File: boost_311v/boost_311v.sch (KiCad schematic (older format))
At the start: 62 parts, among them J1 Vin_Cnt, J2 VO, J3 Vin_boost, Q1 BC556, Q2 PN2222A, Q5 IRFP260, U1 LM358, U2 L7812, U3 TC4420CPA, U4 LF357, U5 NE555

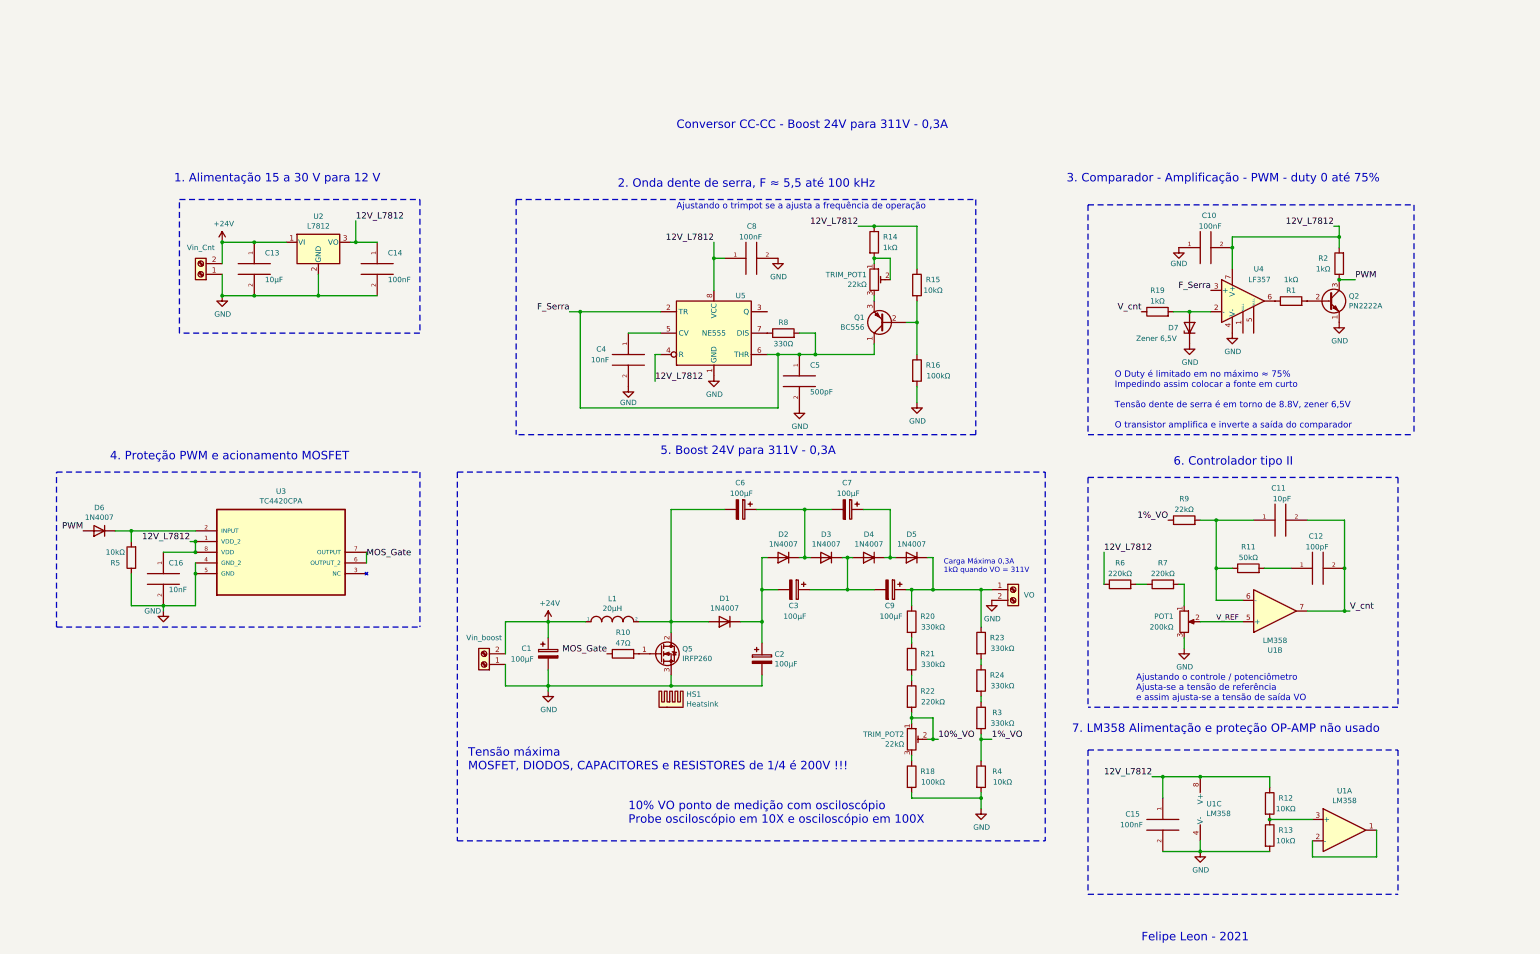
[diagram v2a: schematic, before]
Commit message: UP ocbs
Signed-off-by: fgl27 <fglfgl27@gmail.com>
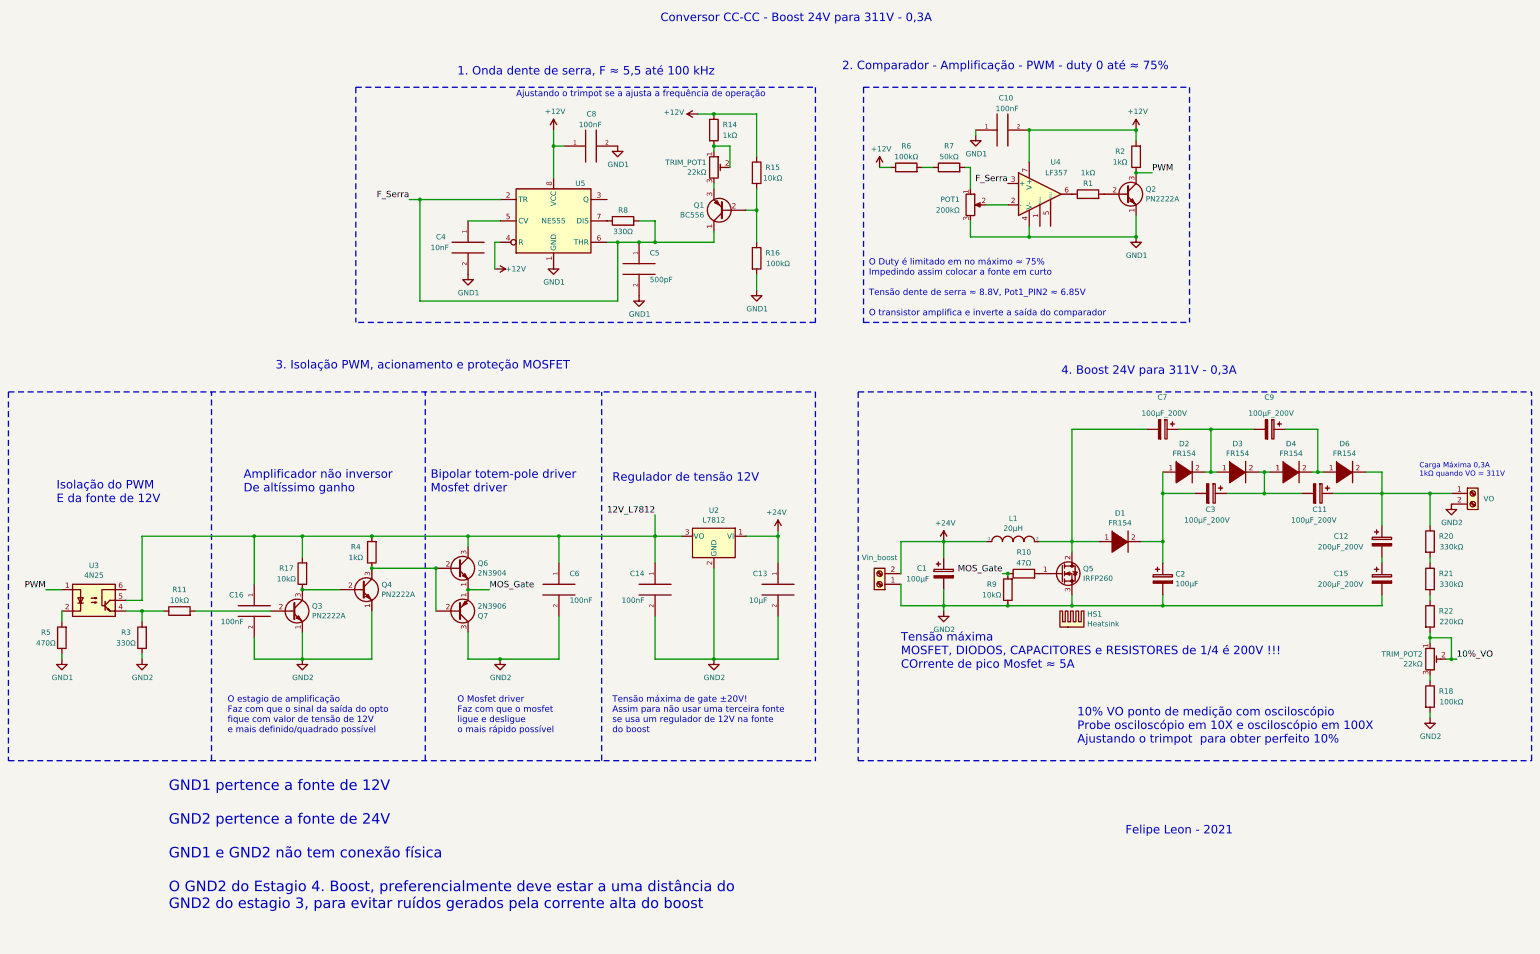
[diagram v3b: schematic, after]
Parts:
- removed C11: 10pF, Capacitor_THT:C_Disc_D7.5mm_W5.0mm_P5.00mm, symbol pspice:CAP
- removed C12: 100pF, Capacitor_THT:C_Disc_D7.5mm_W5.0mm_P5.00mm, symbol pspice:CAP
- removed C15: 100nF, Capacitor_THT:C_Disc_D7.5mm_W5.0mm_P5.00mm, symbol pspice:CAP
- removed C6: 100µF, Capacitor_THT:CP_Radial_D18.0mm_P7.50mm, symbol Device:CP
- removed D1, D2, D3, D4, D5, D6: 1N4007, Diode_THT:D_DO-41_SOD81_P10.16mm_Horizontal, symbol Diode:1N4007
- removed D7: Zener 6,5V, symbol Device:D_Zener
- removed J1: Vin_Cnt, symbol Connector:Screw_Terminal_01x02
- removed R12: 10KΩ, Resistor_THT:R_Axial_DIN0207_L6.3mm_D2.5mm_P10.16mm_Horizontal, symbol Device:R
- removed R13: 10kΩ, Resistor_THT:R_Axial_DIN0207_L6.3mm_D2.5mm_P10.16mm_Horizontal, symbol Device:R
- removed R19: 1kΩ, Resistor_THT:R_Axial_DIN0207_L6.3mm_D2.5mm_P10.16mm_Horizontal, symbol Device:R
- removed R23, R24: 330kΩ, Resistor_THT:R_Axial_DIN0207_L6.3mm_D2.5mm_P10.16mm_Horizontal, symbol Device:R
- removed U1: LM358, symbol Amplifier_Operational:LM358
- removed U3: TC4420CPA, DIP254P762X533-8, symbol 4420:TC4420CPA
- added C11: 100µF_200V, Capacitor_THT:CP_Radial_D18.0mm_P7.50mm, symbol Device:CP
- added C12, C15: 200µF_200V, Capacitor_THT:CP_Radial_D18.0mm_P7.50mm, symbol Device:CP
- added C6: 100nF, Capacitor_THT:C_Disc_D7.5mm_W5.0mm_P5.00mm, symbol pspice:CAP
- added D1, D2, D3, D4, D6: FR154, Diode_THT:D_DO-41_SOD81_P10.16mm_Horizontal, symbol pspice:DIODE
- added Q3, Q4: PN2222A, Package_TO_SOT_THT:TO-92_Inline, symbol Transistor_BJT:PN2222A
- added Q6: 2N3904, Package_TO_SOT_THT:TO-92_Inline, symbol Transistor_BJT:2N3904
- added Q7: 2N3906, Package_TO_SOT_THT:TO-92_Inline, symbol Transistor_BJT:2N3906
- added R17: 10kΩ, Resistor_THT:R_Axial_DIN0207_L6.3mm_D2.5mm_P10.16mm_Horizontal, symbol Device:R
- added U3: 4N25, Package_DIP:DIP-6_W7.62mm, symbol Isolator:4N25
- C16: value 10nF -> 100nF
- C3, C7, C9: value 100µF -> 100µF_200V
- R11: value 50kΩ -> 10kΩ
- R3: value 330kΩ -> 330Ω
- R4: value 10kΩ -> 1kΩ
- R5: value 10kΩ -> 470Ω
- R6: value 220kΩ -> 100kΩ
- R7: value 220kΩ -> 50kΩ
- R9: value 22kΩ -> 10kΩ
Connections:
- net V_REF is gone; now on an unnamed net: POT1.2
- net 12V_L7812: now also R4.2, C6.1, Q6.3 (C), R17.2, U3.5; no longer C10.2, C8.1, R14.1, R15.1, R2.2, R6.1, U4.7 (V+), U5.4 (R), U5.8 (VCC)
- net MOS_Gate: now also R9.2, Q6.1 (E), Q7.1 (E)
- net PWM: now also U3.1
- net at C2.1, C3.2: now also D1.2 (A), D2.1 (K)
- net at L1.2, Q5.2 (D): now also C7.2, D1.1 (K)
- net at C3.1: now also C11.2, D3.2 (A), D4.1 (K); no longer C9.2
- net at C7.1: now also C9.2, D2.2 (A), D3.1 (K)
- net at J2.1 (Pin_1), R20.1: now also C11.1, C12.1, D6.2 (A); no longer C9.1
- net at R5.2: now also U3.2
- net at R11.1: now also R3.2, U3.4; no longer R9.2
- net GND2: now reaches R3.1
- net GND2: now also C1.2, C13.2, C14.2, C16.2, C2.2, J2.2 (Pin_2), J3.1 (Pin_1), Q5.3 (S), R18.2, R9.1, U2.2 (GND), C15.2, C6.2, Q3.1 (E), Q4.1 (E), Q7.3 (C)
- net at R11.2: now also Q3.2 (B)
- removed net 1%_VO: R3.2, R4.1, R9.1
- removed net GND: C1.2, C10.1, C13.2, C14.2, C16.2, C2.2, C4.2, C5.2, C8.2, J2.2 (Pin_2), J3.1 (Pin_1), POT1.3, Q2.1 (E), Q5.3 (S), R16.2, R18.2, R4.2, R5.1, U2.2 (GND), U4.4 (V-), U5.1 (GND)
- new net: Q3.3 (C), Q4.2 (B), R17.1
- new net: Q4.3 (C), Q6.2 (B), Q7.2 (B), R4.1
- new net: C12.2, C15.1
- new net: C9.1, D4.2 (A), D6.1 (K)
- new net +12V: C10.2, C8.1, R14.1, R15.1, R2.2, R6.1, U4.7 (V+), U5.4 (R), U5.8 (VCC)
- new net GND1: C10.1, C4.2, C5.2, C8.2, POT1.3, Q2.1 (E), R16.2, R5.1, U4.4 (V-), U5.1 (GND)
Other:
- note added: "1. Onda dente de serra, F ≈ 5,5 até 100 kHz"
- note added: "10% VO ponto de medição com osciloscópio\nProbe osciloscópio em 10X e osciloscópio em 100X\nAjustando o trimpot para obter perfeito 10%"
- note added: "2. Comparador - Amplificação - PWM - duty 0 até ≈ 75%"
- note added: "3. Isolação PWM, acionamento e proteção MOSFET"
- note added: "4. Boost 24V para 311V - 0,3A"
- note added: "Amplificador não inversor\nDe altíssimo ganho"
- note added: "Bipolar totem-pole driver\nMosfet driver"
- note added: "GND1 pertence a fonte de 12V\n\nGND2 pertence a fonte de 24V\n\nGND1 e GND2 não tem conexão física\n\nO GND2 do Estagio 4. Boost, preferencialmente deve estar a uma distância do\nGND2 do estagio 3, para evitar ruídos gerados pela corrente alta do boost"
- note added: "Isolação do PWM\nE da fonte de 12V"
- note added: "O Duty é limitado em no máximo ≈ 75%\nImpedindo assim colocar a fonte em curto\n\nTensão dente de serra ≈ 8.8V, Pot1_PIN2 ≈ 6.85V\n\nO transistor amplifica e inverte a saída do comparador"
- note added: "O Mosfet driver\nFaz com que o mosfet\nligue e desligue\no mais rápido possível"
- note added: "O estagio de amplificação\nFaz com que o sinal da saída do opto\nfique com valor de tensão de 12V\ne mais definido/quadrado possível"
- note added: "Regulador de tensão 12V"
- note added: "Tensão máxima de gate ±20V!\nAssim para não usar uma terceira fonte\nse usa um regulador de 12V na fonte\ndo boost"
- note added: "Tensão máxima\nMOSFET, DIODOS, CAPACITORES e RESISTORES de 1/4 é 200V !!!\nCOrrente de pico Mosfet ≈ 5A"
- note removed: "1. Alimentação 15 a 30 V para 12 V"
- note removed: "10% VO ponto de medição com osciloscópio\nProbe osciloscópio em 10X e osciloscópio em 100X"
- note removed: "2. Onda dente de serra, F ≈ 5,5 até 100 kHz"
- note removed: "3. Comparador - Amplificação - PWM - duty 0 até 75%"
- note removed: "4. Proteção PWM e acionamento MOSFET"
- note removed: "5. Boost 24V para 311V - 0,3A"
- note removed: "6. Controlador tipo II"
- note removed: "7. LM358 Alimentação e proteção OP-AMP não usado"
- note removed: "Ajustando o controle / potenciômetro\nAjusta-se a tensão de referência\ne assim ajusta-se a tensão de saída VO"
- note removed: "O Duty é limitado em no máximo ≈ 75%\nImpedindo assim colocar a fonte em curto\n\nTensão dente de serra é em torno de 8.8V, zener 6,5V\n\nO transistor amplifica e inverte a saída do comparador"
- note removed: "Tensão máxima\nMOSFET, DIODOS, CAPACITORES e RESISTORES de 1/4 é 200V !!!"
- moved on the sheet: C1, C10, C13, C14, C2, C3, C4, C5, C8, HS1, L1, POT1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
